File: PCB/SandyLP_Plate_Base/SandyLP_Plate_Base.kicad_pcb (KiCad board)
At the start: 2 copper layers, 285 x 84.3 mm, 1 part

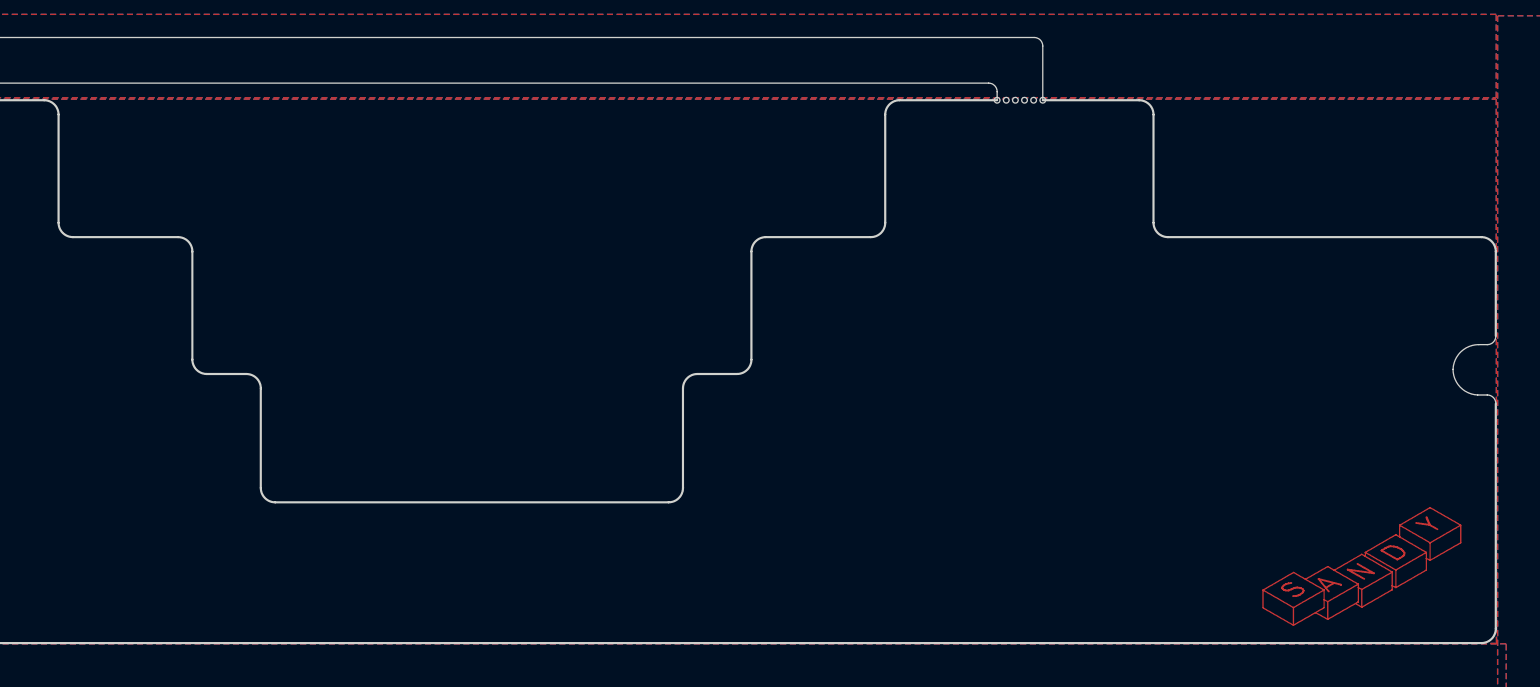
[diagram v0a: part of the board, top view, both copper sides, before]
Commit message: ロゴ追加
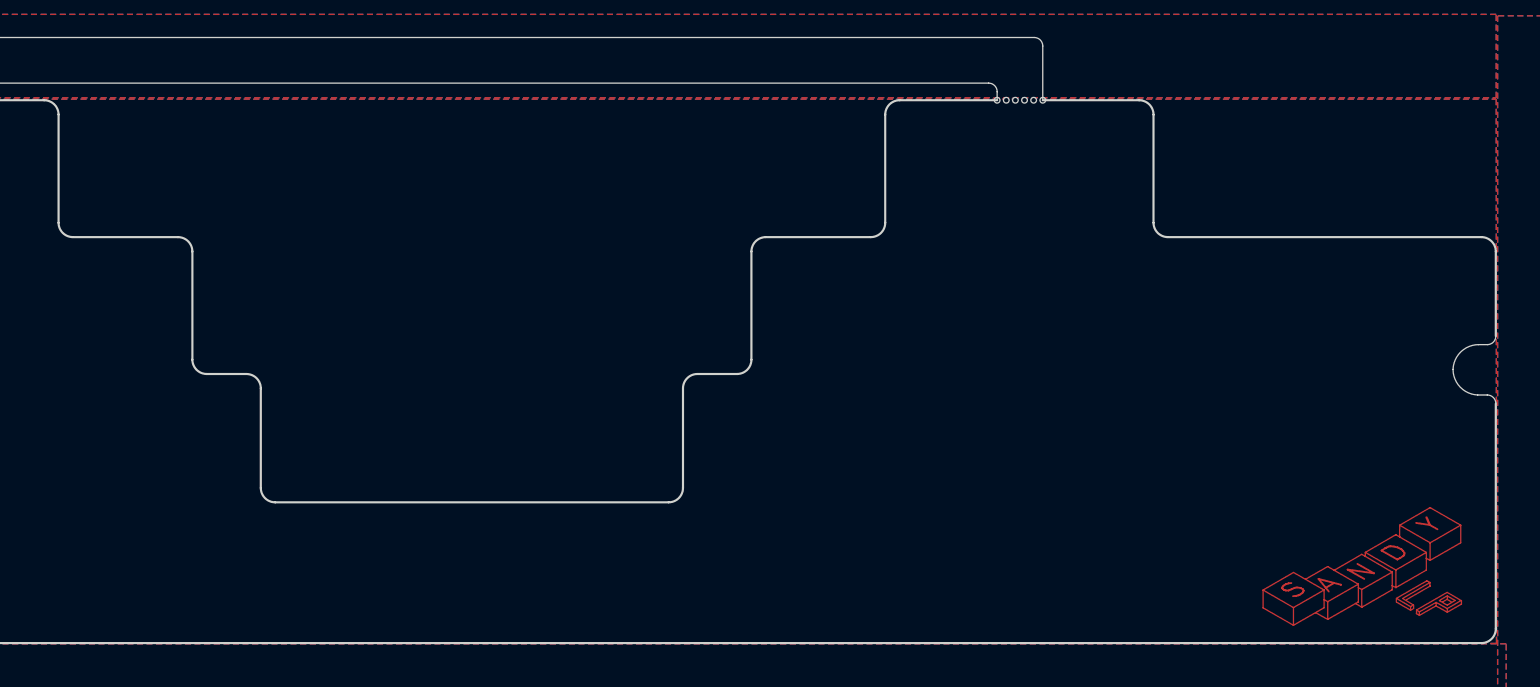
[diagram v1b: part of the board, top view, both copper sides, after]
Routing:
- net (no net): track 187.8 -> 240.9 mm

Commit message: 外形調整。スイッチ穴配置。
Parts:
- added SW_/1: SW_Push, locallib:MX-Switch-Hole-with-narrow-frame, F.Cu at (274.3, 84.3)
- added SW_;1: SW_Push, locallib:MX-Switch-Hole-with-narrow-frame, F.Cu at (264.8, 65.2)
- added SW_<1: SW_Push, locallib:MX-Switch-Hole-with-narrow-frame, F.Cu at (236.2, 84.3)
- added SW_>1: SW_Push, locallib:MX-Switch-Hole-with-narrow-frame, F.Cu at (255.2, 84.3)
- added SW_A1: SW_Push, locallib:MX-Switch-Hole-with-narrow-frame, F.Cu at (55.2, 65.2)
- added SW_B1: SW_Push, locallib:MX-Switch-Hole-with-narrow-frame, F.Cu at (121.9, 84.3)
- added SW_C1: SW_Push, locallib:MX-Switch-Hole-with-narrow-frame, F.Cu at (83.8, 84.3)
- added SW_CTL1: SW_Push, locallib:MX-Switch-Hole-with-narrow-frame, F.Cu at (36.2, 65.2)
- added SW_D1: SW_Push, locallib:MX-Switch-Hole-with-narrow-frame, F.Cu at (93.3, 65.2)
- added SW_E1: SW_Push, locallib:MX-Switch-Hole-with-narrow-frame, F.Cu at (93.3, 46.2)
- added SW_ENT1: SW_Push, locallib:MX-Switch-Hole-with-narrow-frame, F.Cu at (283.8, 65.2)
- added SW_F1: SW_Push, locallib:MX-Switch-Hole-with-narrow-frame, F.Cu at (112.4, 65.2)
- added SW_I1: SW_Push, locallib:MX-Switch-Hole-with-narrow-frame, F.Cu at (226.7, 46.2)
- added SW_J1: SW_Push, locallib:MX-Switch-Hole-with-narrow-frame, F.Cu at (207.6, 65.2)
- added SW_K1: SW_Push, locallib:MX-Switch-Hole-with-narrow-frame, F.Cu at (226.7, 65.2)
- added SW_L1: SW_Push, locallib:MX-Switch-Hole-with-narrow-frame, F.Cu at (245.7, 65.2)
- added SW_LALTu1: SW_Push, locallib:MX-Switch-Hole-with-narrow-frame, F.Cu at (98.1, 103.3)
- added SW_LSPC1: SW_Push, locallib:MX-Switch-Hole-with-narrow-frame, F.Cu at (119.5, 103.3)
- added SW_LWIN1: SW_Push, locallib:MX-Switch-Hole-with-narrow-frame, F.Cu at (79.0, 103.3)
- added SW_M1: SW_Push, locallib:MX-Switch-Hole-with-narrow-frame, F.Cu at (217.1, 84.3)
- added SW_N1: SW_Push, locallib:MX-Switch-Hole-with-narrow-frame, F.Cu at (198.1, 84.3)
- added SW_O1: SW_Push, locallib:MX-Switch-Hole-with-narrow-frame, F.Cu at (245.7, 46.2)
- added SW_R5CNT_C1: RotaryEncoder_Switch, locallib:MX-Switch-Hole-with-narrow-frame, F.Cu at (160.0, 103.3)
- added SW_R5CNT_L1: SW_Push, locallib:MX-Switch-Hole-with-narrow-frame, F.Cu at (140.9, 103.3)
- added SW_R5CNT_R1: SW_Push, locallib:MX-Switch-Hole-with-narrow-frame, F.Cu at (179.0, 103.3)
- added SW_RALT1: SW_Push, locallib:MX-Switch-Hole-with-narrow-frame, F.Cu at (221.9, 103.3)
- added SW_RSPC1: SW_Push, locallib:MX-Switch-Hole-with-narrow-frame, F.Cu at (200.5, 103.3)
- added SW_RWIN1: SW_Push, locallib:MX-Switch-Hole-with-narrow-frame, F.Cu at (241.0, 103.3)
- added SW_S1: SW_Push, locallib:MX-Switch-Hole-with-narrow-frame, F.Cu at (74.3, 65.2)
- added SW_V1: SW_Push, locallib:MX-Switch-Hole-with-narrow-frame, F.Cu at (102.8, 84.3)
- added SW_W1: SW_Push, locallib:MX-Switch-Hole-with-narrow-frame, F.Cu at (74.3, 46.2)
- added SW_X1: SW_Push, locallib:MX-Switch-Hole-with-narrow-frame, F.Cu at (64.7, 84.3)
- added SW_Z1: SW_Push, locallib:MX-Switch-Hole-with-narrow-frame, F.Cu at (45.7, 84.3)
- REF**: footprint locallib:60_Outline-Sandy-DN0040-Plate-Base-sw-hole -> locallib:SandyLP_outline_Plate_Base_small_panel
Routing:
- net (no net): track 240.9 -> 237.9 mm
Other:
- board size 285 x 84.3 mm -> 275.5 x 80.3 mm
- board text added: "#SandyLP_kbd DN0010, Plate for Base by @jpskenn"
- board text removed: "#Sandy_kbd DN0040, Plate for Base by @jpskenn"
- board text removed: "Back Side"
- board text removed: "KEEP AWAY from CUT LINE"
